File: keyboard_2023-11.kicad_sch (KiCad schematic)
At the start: 76 parts, among them J1 Conn_01x04, J10 Conn_01x01_Socket, J11 Conn_01x07_Socket, J2 Conn_01x04_Socket, J3 Conn_01x07_Socket, J4 Conn_01x07_Pin, J5 Conn_01x01_Socket, J6 Conn_01x01_Socket, J7 Conn_01x01_Socket, J8 Conn_01x01_Socket, J9 Conn_01x01_Socket, SW1 SW_Push, SW10 SW_Push, SW11 SW_Push, SW12 SW_Push, SW13 SW_Push, SW14 SW_Push, SW15 SW_Push, SW16 SW_Push, SW17 SW_Push, SW18 SW_Push, SW19 SW_Push, SW2 SW_Push, SW20 SW_Push, SW21 SW_Push, SW22 SW_Push, SW23 SW_Push, SW24 SW_Push, SW3 SW_Push, SW4 SW_Push, SW5 SW_Push, SW6 SW_Push, SW7 SW_Push, SW8 SW_Push, SW9 SW_Push, U1 MCP23017_SO, U2 MCP23017_SO

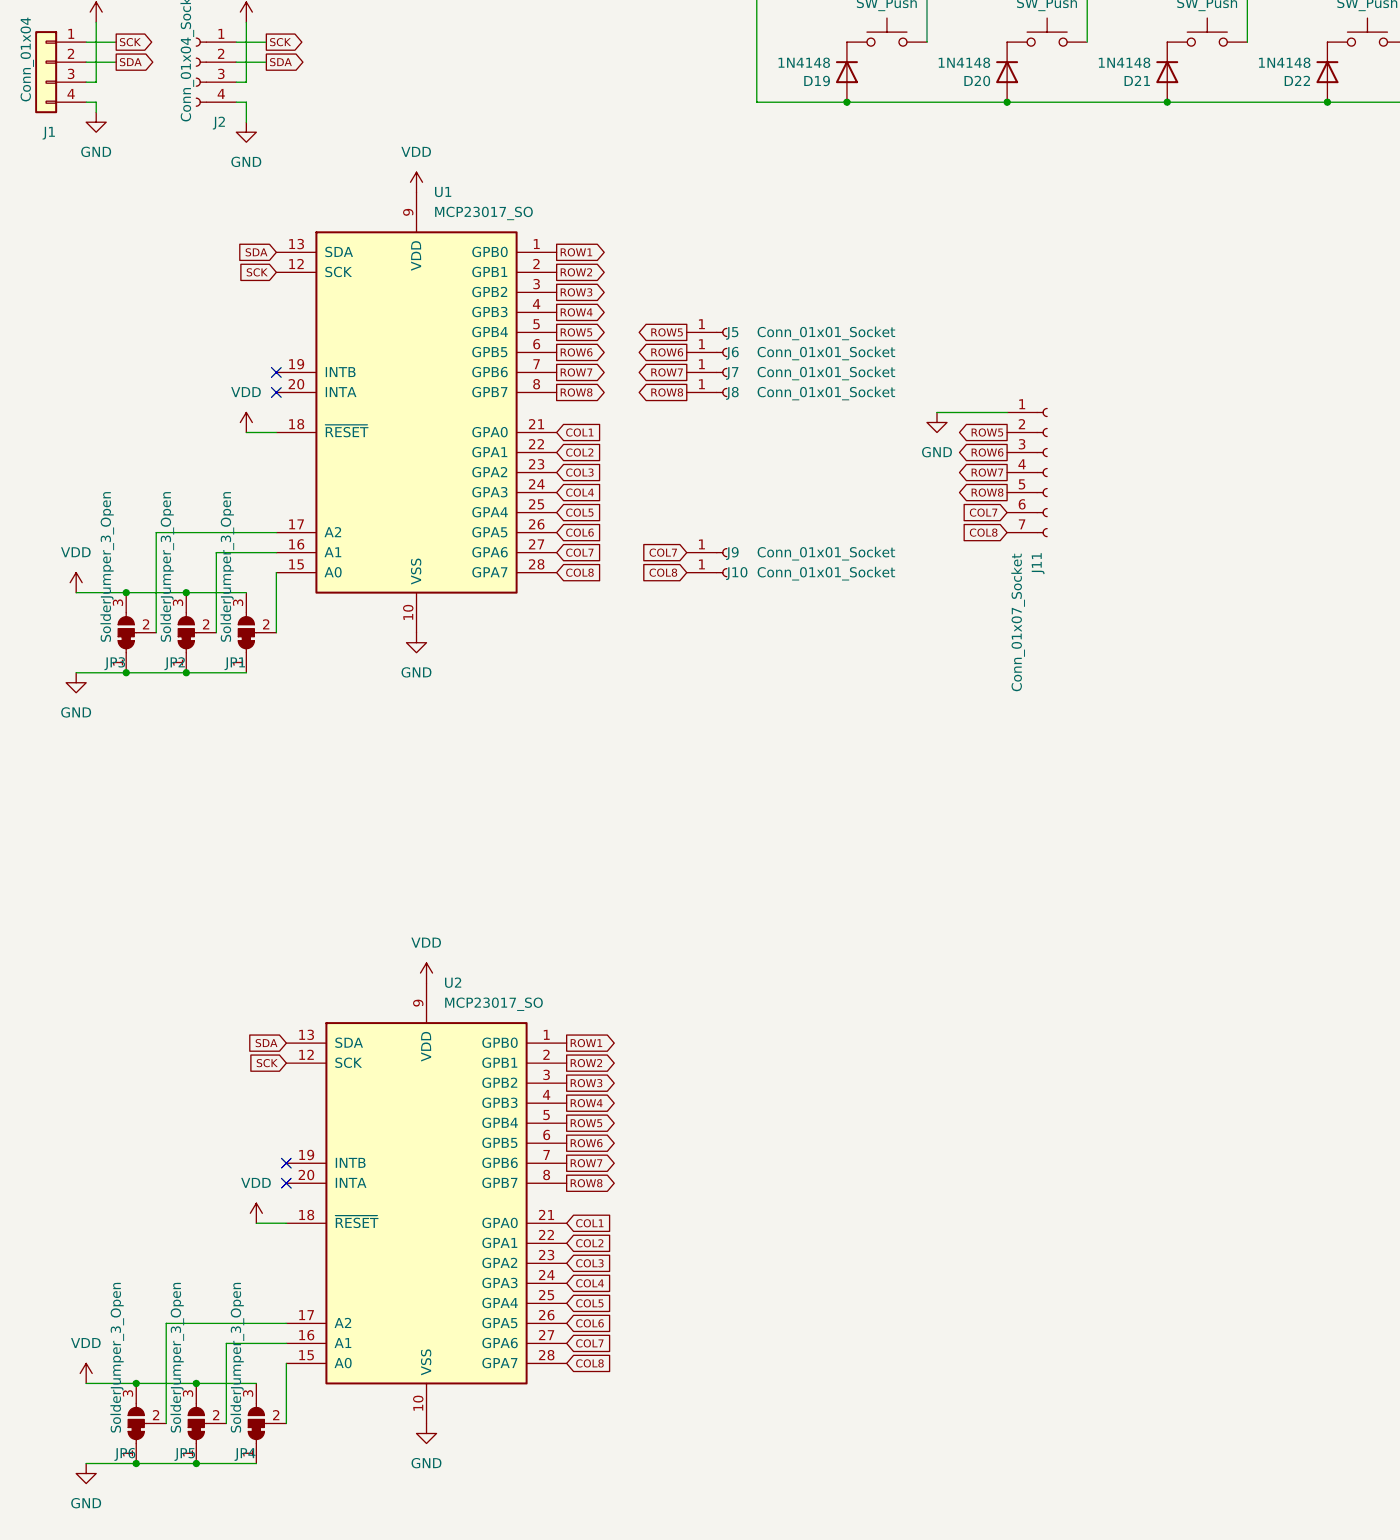
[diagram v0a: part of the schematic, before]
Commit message: routed 90%
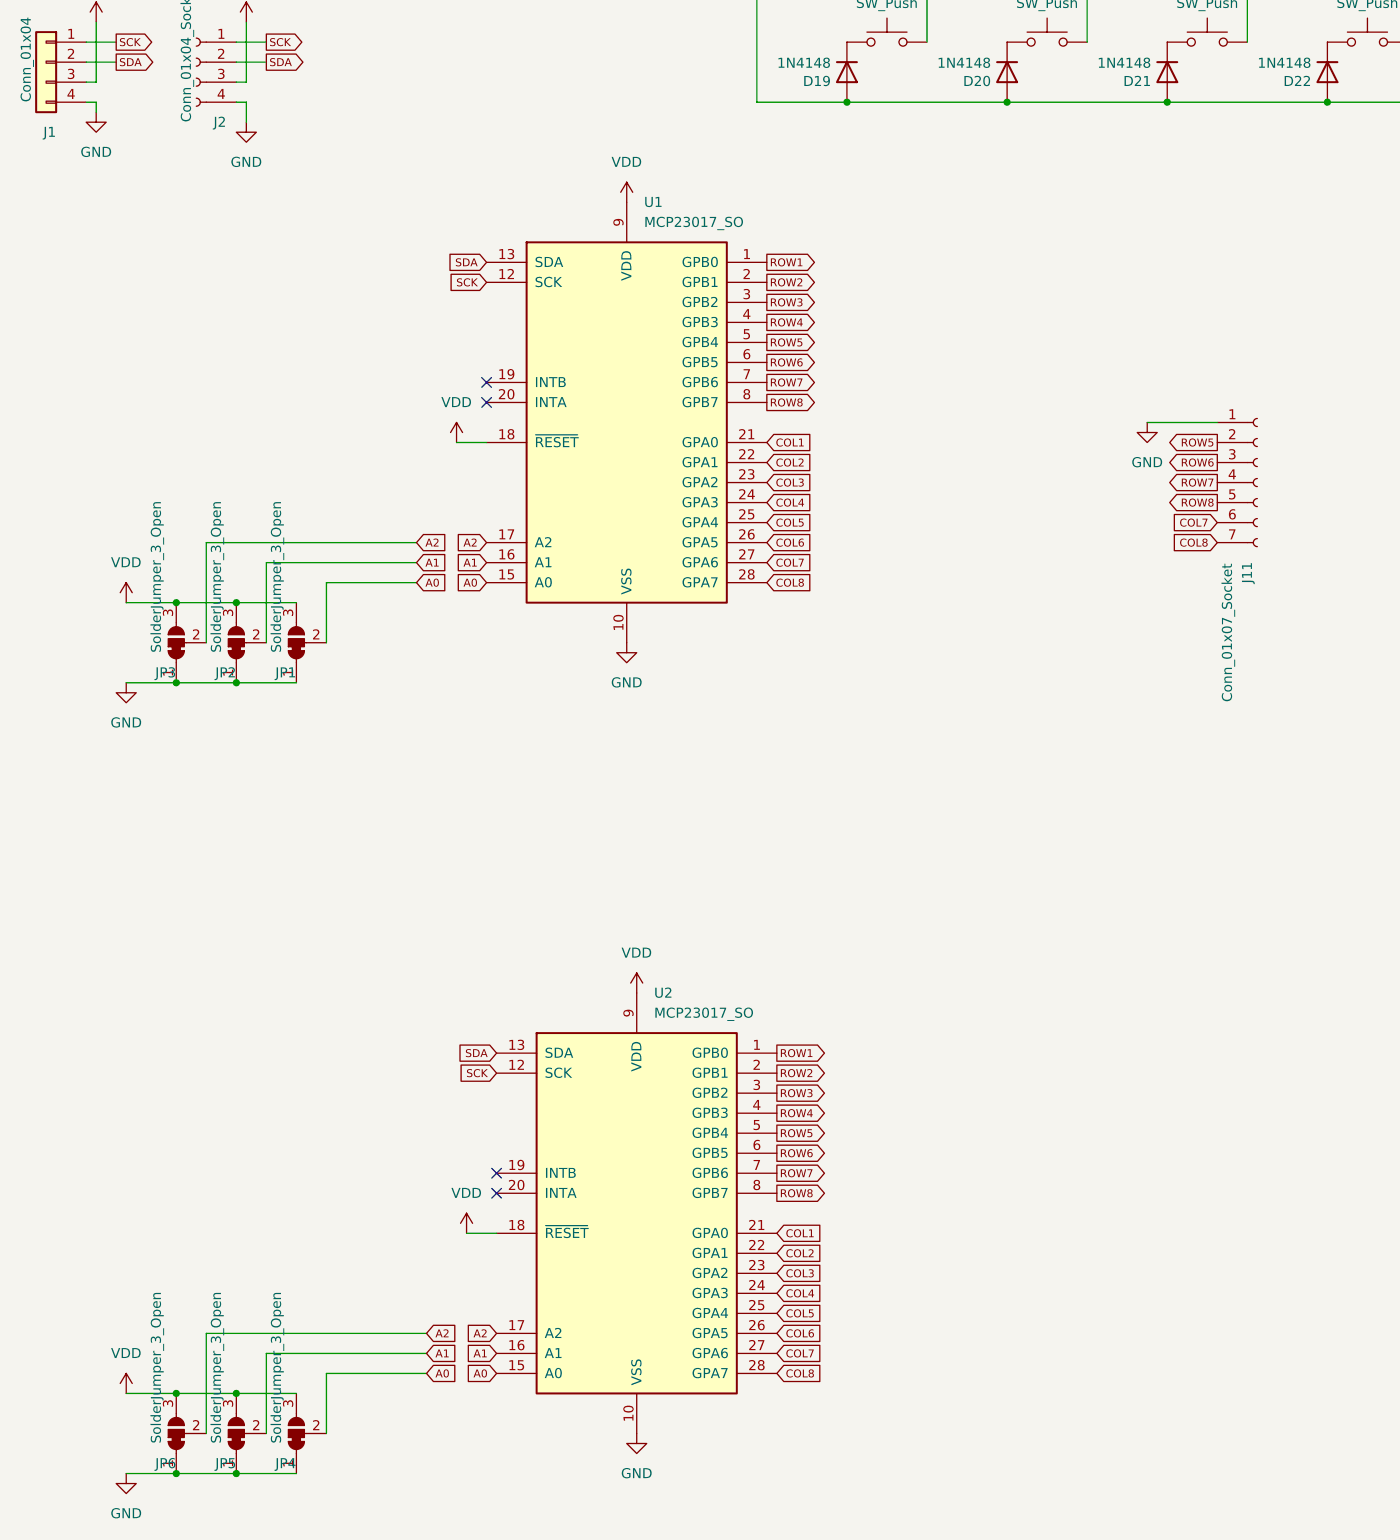
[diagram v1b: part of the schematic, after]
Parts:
- removed J10, J5, J6, J7, J8, J9: Conn_01x01_Socket, project-local:PinHeader_1x01_P2.54mm_Vertical, symbol Connector:Conn_01x01_Socket
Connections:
- net A0: now reaches JP4.2 (C), U2.15 (A0)
- net A0: now also JP1.2 (C), U1.15 (A0)
- net A1: now reaches JP2.2 (C), U1.16 (A1)
- net A1: now also JP5.2 (C), U2.16 (A1)
- net A2: now reaches JP3.2 (C), U1.17 (A2)
- net A2: now also JP6.2 (C), U2.17 (A2)
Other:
- moved on the sheet: J11, JP1, JP2, JP3, JP4, JP5, JP6, U1, U2

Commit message: snapshot
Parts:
- SW1, SW10, SW11, SW12, SW13, SW14, SW15, SW16, SW17, SW18, SW19, SW2, SW20, SW21, SW22, SW23, SW24, SW3, SW4, SW5, SW6, SW7, SW8, SW9: footprint keyswitches:SW_MX_reversible -> project-local:SW_MX_reversible
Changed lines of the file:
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@@
       (effects (font (size 1.27 1.27)))
     )
-    (property "Footprint" "keyswitches:SW_MX_reversible" (at 124.46 60.96 0)
+    (property "Footprint" "project-local:SW_MX_reversible" (at 124.46 60.96 0)
       (effects (font (size 1.27 1.27)) hide)
     )
@@
       (effects (font (size 1.27 1.27)))
     )
-    (property "Footprint" "keyswitches:SW_MX_reversible" (at 124.46 43.18 0)
+    (property "Footprint" "project-local:SW_MX_reversible" (at 124.46 43.18 0)
       (effects (font (size 1.27 1.27)) hide)
     )
@@
       (effects (font (size 1.27 1.27)))
     )
-    (property "Footprint" "keyswitches:SW_MX_reversible" (at 185.42 60.96 0)
+    (property "Footprint" "project-local:SW_MX_reversible" (at 185.42 60.96 0)
       (effects (font (size 1.27 1.27)) hide)
     )
@@
       (effects (font (size 1.27 1.27)))
     )
-    (property "Footprint" "keyswitches:SW_MX_reversible" (at 165.1 43.18 0)
+    (property "Footprint" "project-local:SW_MX_reversible" (at 165.1 43.18 0)
       (effects (font (size 1.27 1.27)) hide)
     )
@@
       (effects (font (size 1.27 1.27)))
     )
-    (property "Footprint" "keyswitches:SW_MX_reversible" (at 124.46 100.33 0)
+    (property "Footprint" "project-local:SW_MX_reversible" (at 124.46 100.33 0)
       (effects (font (size 1.27 1.27)) hide)
     )
@@
       (effects (font (size 1.27 1.27)))
     )
-    (property "Footprint" "keyswitches:SW_MX_reversible" (at 124.46 24.13 0)
+    (property "Footprint" "project-local:SW_MX_reversible" (at 124.46 24.13 0)
       (effects (font (size 1.27 1.27)) hide)
     )
@@
       (effects (font (size 1.27 1.27)))
     )
-    (property "Footprint" "keyswitches:SW_MX_reversible" (at 144.78 60.96 0)
+    (property "Footprint" "project-local:SW_MX_reversible" (at 144.78 60.96 0)
       (effects (font (size 1.27 1.27)) hide)
     )
@@
       (effects (font (size 1.27 1.27)))
     )
-    (property "Footprint" "keyswitches:SW_MX_reversible" (at 226.06 100.33 0)
+    (property "Footprint" "project-local:SW_MX_reversible" (at 226.06 100.33 0)
       (effects (font (size 1.27 1.27)) hide)
     )
@@
       (effects (font (size 1.27 1.27)))
     )
-    (property "Footprint" "keyswitches:SW_MX_reversible" (at 226.06 60.96 0)
+    (property "Footprint" "project-local:SW_MX_reversible" (at 226.06 60.96 0)
       (effects (font (size 1.27 1.27)) hide)
     )
@@
       (effects (font (size 1.27 1.27)))
     )
-    (property "Footprint" "keyswitches:SW_MX_reversible" (at 205.74 100.33 0)
+    (property "Footprint" "project-local:SW_MX_reversible" (at 205.74 100.33 0)
       (effects (font (size 1.27 1.27)) hide)
     )
@@
       (effects (font (size 1.27 1.27)))
     )
-    (property "Footprint" "keyswitches:SW_MX_reversible" (at 144.78 24.13 0)
+    (property "Footprint" "project-local:SW_MX_reversible" (at 144.78 24.13 0)
       (effects (font (size 1.27 1.27)) hide)
     )
@@
       (effects (font (size 1.27 1.27)))
     )
-    (property "Footprint" "keyswitches:SW_MX_reversible" (at 226.06 43.18 0)
+    (property "Footprint" "project-local:SW_MX_reversible" (at 226.06 43.18 0)
       (effects (font (size 1.27 1.27)) hide)
     )
@@
       (effects (font (size 1.27 1.27)))
     )
-    (property "Footprint" "keyswitches:SW_MX_reversible" (at 165.1 24.13 0)
+    (property "Footprint" "project-local:SW_MX_reversible" (at 165.1 24.13 0)
       (effects (font (size 1.27 1.27)) hide)
     )
@@
       (effects (font (size 1.27 1.27)))
     )
-    (property "Footprint" "keyswitches:SW_MX_reversible" (at 144.78 43.18 0)
+    (property "Footprint" "project-local:SW_MX_reversible" (at 144.78 43.18 0)
       (effects (font (size 1.27 1.27)) hide)
     )
@@
       (effects (font (size 1.27 1.27)))
     )
-    (property "Footprint" "keyswitches:SW_MX_reversible" (at 226.06 24.13 0)
+    (property "Footprint" "project-local:SW_MX_reversible" (at 226.06 24.13 0)
       (effects (font (size 1.27 1.27)) hide)
     )
@@
       (effects (font (size 1.27 1.27)))
     )
-    (property "Footprint" "keyswitches:SW_MX_reversible" (at 185.42 100.33 0)
+    (property "Footprint" "project-local:SW_MX_reversible" (at 185.42 100.33 0)
       (effects (font (size 1.27 1.27)) hide)
     )
@@
       (effects (font (size 1.27 1.27)))
     )
-    (property "Footprint" "keyswitches:SW_MX_reversible" (at 205.74 24.13 0)
+    (property "Footprint" "project-local:SW_MX_reversible" (at 205.74 24.13 0)
       (effects (font (size 1.27 1.27)) hide)
     )
@@
       (effects (font (size 1.27 1.27)))
     )
-    (property "Footprint" "keyswitches:SW_MX_reversible" (at 144.78 100.33 0)
+    (property "Footprint" "project-local:SW_MX_reversible" (at 144.78 100.33 0)
       (effects (font (size 1.27 1.27)) hide)
     )
@@
       (effects (font (size 1.27 1.27)))
     )
-    (property "Footprint" "keyswitches:SW_MX_reversible" (at 205.74 60.96 0)
+    (property "Footprint" "project-local:SW_MX_reversible" (at 205.74 60.96 0)
       (effects (font (size 1.27 1.27)) hide)
     )
@@
       (effects (font (size 1.27 1.27)))
     )
-    (property "Footprint" "keyswitches:SW_MX_reversible" (at 205.74 43.18 0)
+    (property "Footprint" "project-local:SW_MX_reversible" (at 205.74 43.18 0)
       (effects (font (size 1.27 1.27)) hide)
     )
@@
       (effects (font (size 1.27 1.27)))
     )
-    (property "Footprint" "keyswitches:SW_MX_reversible" (at 185.42 24.13 0)
+    (property "Footprint" "project-local:SW_MX_reversible" (at 185.42 24.13 0)
       (effects (font (size 1.27 1.27)) hide)
     )
@@
       (effects (font (size 1.27 1.27)))
     )
-    (property "Footprint" "keyswitches:SW_MX_reversible" (at 185.42 43.18 0)
+    (property "Footprint" "project-local:SW_MX_reversible" (at 185.42 43.18 0)
       (effects (font (size 1.27 1.27)) hide)
     )
@@
       (effects (font (size 1.27 1.27)))
     )
-    (property "Footprint" "keyswitches:SW_MX_reversible" (at 165.1 100.33 0)
+    (property "Footprint" "project-local:SW_MX_reversible" (at 165.1 100.33 0)
       (effects (font (size 1.27 1.27)) hide)
     )
@@
       (effects (font (size 1.27 1.27)))
     )
-    (property "Footprint" "keyswitches:SW_MX_reversible" (at 165.1 60.96 0)
-      (effects (font (size 1.27 1.27)) hide)
-    )
+    (property "Footprint" "project-local:SW_MX_reversible" (at 165.1 60.96 0)
+      (effects (font (size 1.27 1.27)) hide)
+    )
